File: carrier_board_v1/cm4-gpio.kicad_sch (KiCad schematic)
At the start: 10 parts, among them J1 B2B-PH-SM4-TB_LF__SN_, J2 USB4105-GF-A, U1 MCP73831-2-OT, U2 TPS63061

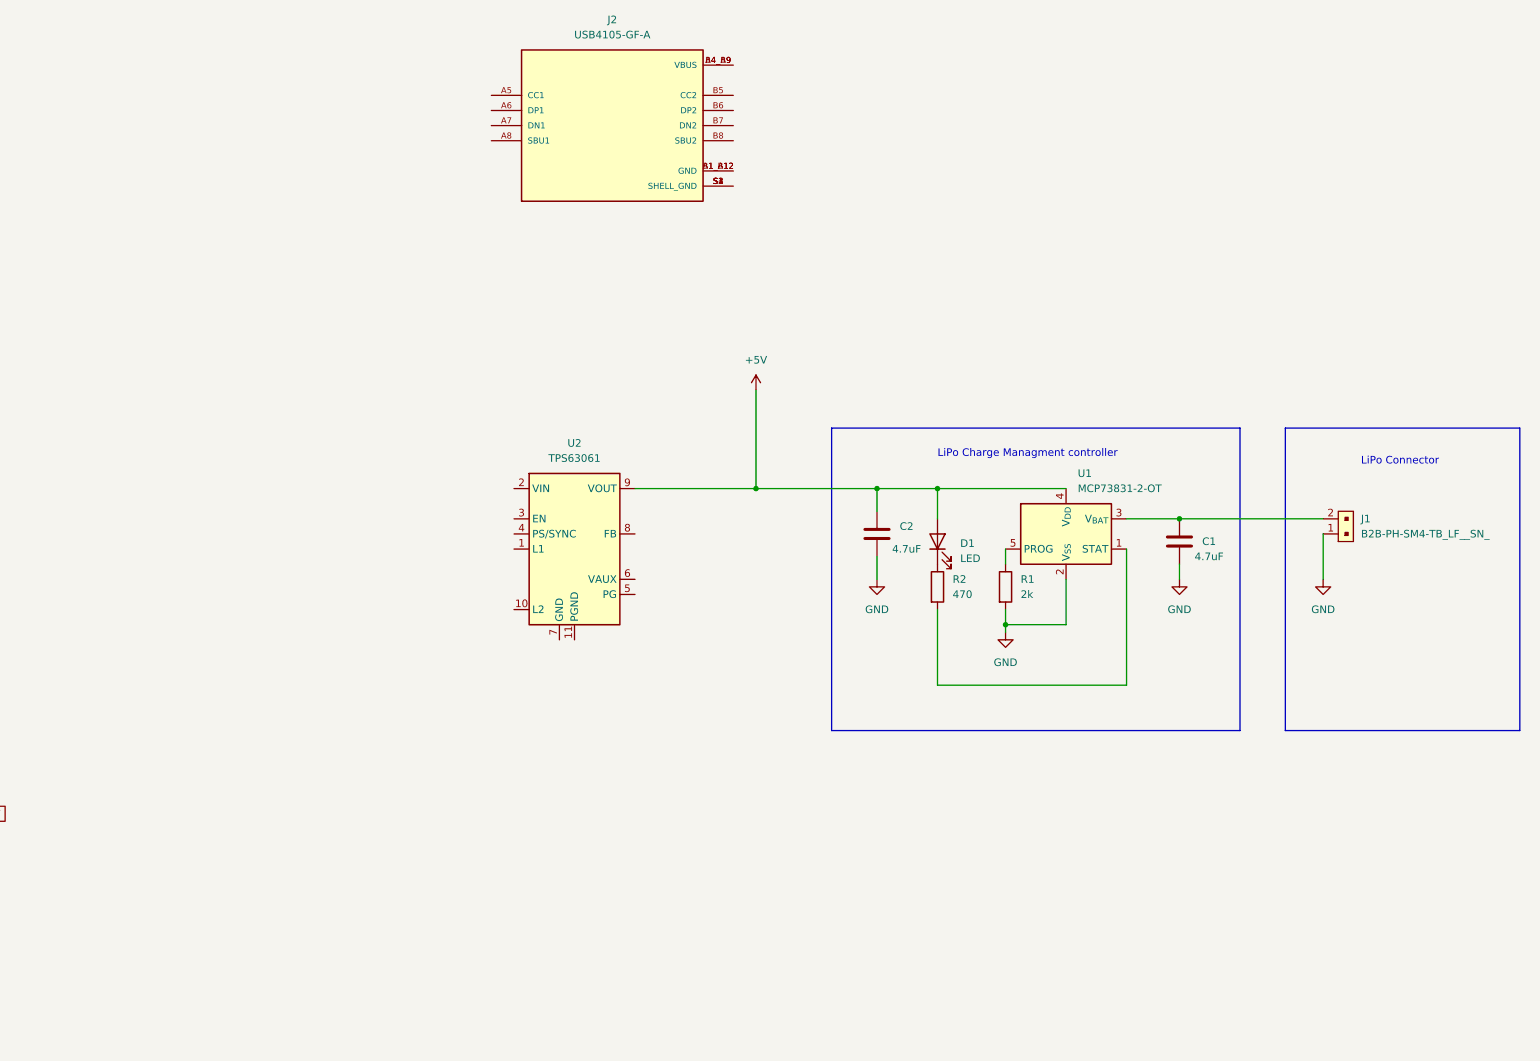
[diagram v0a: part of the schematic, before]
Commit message: -
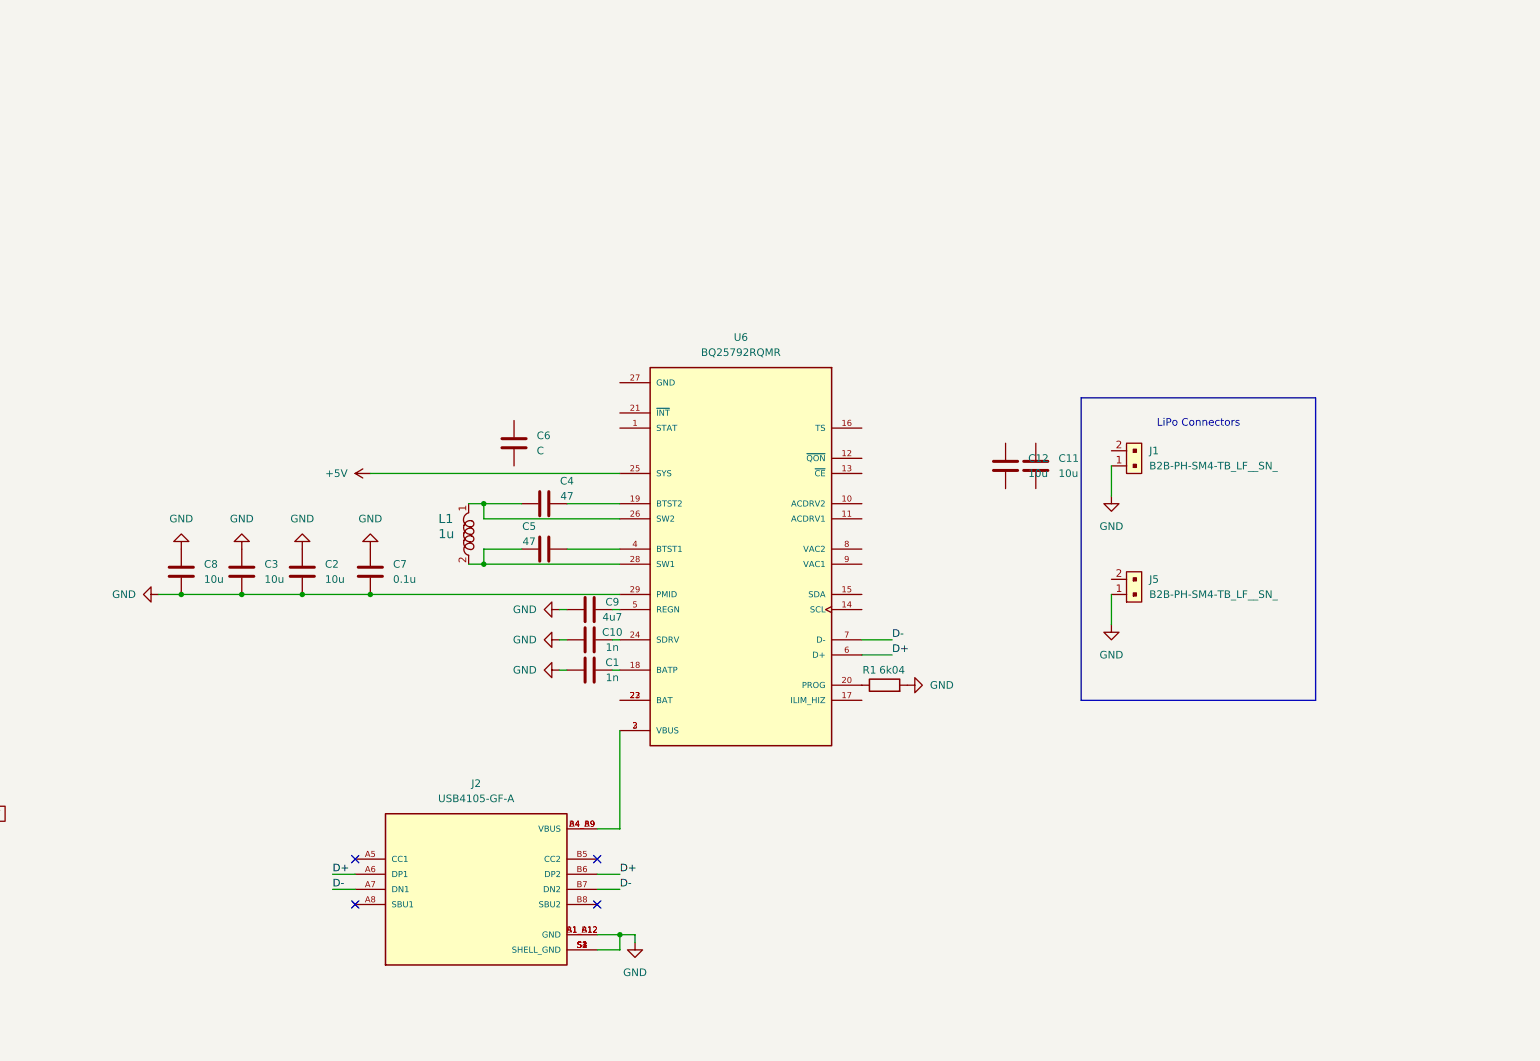
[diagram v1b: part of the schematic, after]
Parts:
- removed D1: LED, symbol Device:LED
- removed R2: 470, symbol Device:R
- removed U1: MCP73831-2-OT, Package_TO_SOT_SMD:SOT-23-5, symbol Battery_Management:MCP73831-2-OT
- removed U2: TPS63061, Package_SON:Texas_S-PWSON-N10_ThermalVias, symbol Regulator_Switching:TPS63061
- added C10: 1n, symbol Device:C
- added C11, C12, C3, C8: 10u, symbol Device:C
- added C4, C5: 47, symbol Device:C
- added C6: C, symbol Device:C
- added C7: 0.1u, symbol Device:C
- added C9: 4u7, symbol Device:C
- added J5: B2B-PH-SM4-TB_LF__SN_, digikey-footprints:PinHeader_1x2_P2mm, symbol dk_Rectangular-Connectors-Headers-Male-Pins:B2B-PH-SM4-TB_LF__SN_
- added L1: 1u, digikey-footprints:1210, symbol dk_Fixed-Inductors:82473C
- added U6: BQ25792RQMR, QFN40P400X400X100-29N, symbol BQ25792RQMR:BQ25792RQMR
- C1: value 4.7uF -> 1n
- C2: value 4.7uF -> 10u
- R1: value 2k -> 6k04
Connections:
- net +5V: now also U6.25 (SYS); no longer C2.1
- net GND: now also C1.1, C2.1, J2.A1_B12 (GND), J2.B1_A12 (GND), J2.S1 (SHELL_GND), J2.S2 (SHELL_GND), J2.S3 (SHELL_GND), J2.S4 (SHELL_GND), C10.1, C3.1, C3.2, C7.1, C7.2, C8.1, C8.2, C9.1, J5.1, U6.29 (PMID); no longer C1.2
- net at R1.1: now also U6.20 (PROG)
- net at J2.A4_B9 (VBUS), J2.B4_A9 (VBUS): now also U6.2 (VBUS), U6.3 (VBUS)
- net D+: now reaches J2.A6 (DP1)
- net D+: now also J2.B6 (DP2), U6.6 (D+)
- net D-: now reaches J2.A7 (DN1)
- net D-: now also J2.B7 (DN2), U6.7 (D-)
- net at J1.2: no longer C1.1
- new net: C4.1, L1.1, U6.26 (SW2)
- new net: C5.2, L1.2, U6.28 (SW1)
- new net: C1.2, U6.18 (BATP)
- new net: C10.2, U6.24 (SDRV)
- new net: C4.2, U6.19 (BTST2)
- new net: U6.22 (BAT), U6.23 (BAT)
- new net: C5.1, U6.4 (BTST1)
- new net: C9.2, U6.5 (REGN)
- no-connect marks 0 -> 4
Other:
- note added: "LiPo Connectors"
- note removed: "LiPo Charge Managment controller"
- note removed: "LiPo Connector"
- moved on the sheet: J1, J2

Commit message: -
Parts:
- removed C10: 1n, symbol Device:C
- removed C3, C8: 10u, symbol Device:C
- removed C4, C5: 47, symbol Device:C
- removed C6: C, symbol Device:C
- removed C7: 0.1u, symbol Device:C
- removed C9: 4u7, symbol Device:C
- removed J2: USB4105-GF-A, GCT_USB4105-GF-A, symbol USB4105-GF-A:USB4105-GF-A
- removed J5: B2B-PH-SM4-TB_LF__SN_, digikey-footprints:PinHeader_1x2_P2mm, symbol dk_Rectangular-Connectors-Headers-Male-Pins:B2B-PH-SM4-TB_LF__SN_
- removed L1: 1u, digikey-footprints:1210, symbol dk_Fixed-Inductors:82473C
- removed R1: 6k04, symbol Device:R
- removed U6: BQ25792RQMR, QFN40P400X400X100-29N, symbol BQ25792RQMR:BQ25792RQMR
- added C17, C18, C19: 22u, symbol Device:C
- added J6: USB4105-GF-A, GCT_USB4105-GF-A, symbol USB4105-GF-A:USB4105-GF-A
- added L2: 1.5u, digikey-footprints:Inductor_13R106C, symbol dk_Fixed-Inductors:13R106C
- added L3: 1u, digikey-footprints:Inductor_13R106C, symbol dk_Fixed-Inductors:13R106C
- added R10: 1k, symbol Device:R
- added R11: 150k, symbol Device:R
- added R9: 2k, symbol Device:R
- added U1: MP2624GL-P, QFN-22_MP2624_MNP, symbol MP2624:MP2624GL-P
- added U2: MP3423GG-P, QFN14_MP3423_MNP, symbol MP3423:MP3423GG-P
- C1: value 1n -> 22u
- C11: value 10u -> 4.7u
- C12, C2: value 10u -> 22u
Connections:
- net +5V: now also C1.1, C2.1, U2.4 (OUT), U2.5 (OUT), U2.6 (OUT)
- net GND: now also C11.1, C12.1, J6.A1_B12 (GND), J6.B1_A12 (GND), J6.S1 (SHELL_GND), J6.S2 (SHELL_GND), J6.S3 (SHELL_GND), J6.S4 (SHELL_GND), R11.1, U1.5 (PGND); no longer C1.1, C2.1, C2.2
- net GNDD: now reaches C1.2
- net GNDD: now also C2.2, C17.2, C18.2, C19.2, U2.1 (PGND), U2.11 (AGND), U2.13 (PGND), U2.2 (PGND)
- net at C11.2: now also U1.3 (PMID)
- net at J1.2: now also C12.2, U1.16 (BATT)
- new net: R11.2, U2.12 (FB)
- new net: R10.2, U1.20 (*STAT)
- new net: L2.1, U2.14 (SW), U2.3 (SW)
- new net: R9.1, U1.21 (INT)
- new net: J6.A4_B9 (VBUS), J6.B4_A9 (VBUS), U1.2 (IN)
- new net DN: J6.A7 (DN1), J6.B7 (DN2), U1.22 (DM)
- new net DP: J6.A6 (DP1), J6.B6 (DP2), U1.1 (DP)
- new net EN: U2.8 (EN)
- new net GPIO_VREF: R10.1, R9.2
- new net SW: L3.1, U1.14 (SW), U1.4 (SW)
- new net SYS: C17.1, C18.1, C19.1, L2.2, L3.2, U1.15 (SYS), U2.10 (INA), U2.9 (IN)
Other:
- note added: "LiPo battery charger IC (MP2624)"
- note added: "USB C"
- note added: "Voltage step-up converter (MP3423)"
- moved on the sheet: J1, Module1A
